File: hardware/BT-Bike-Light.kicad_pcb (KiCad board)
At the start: 4 copper layers, 35 x 80 mm, 46 parts, among them J101 USB_C_Charge_Port, J102 Conn_ARM_SWD_TagConnect_TC203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, J103 BATT, Q101 DMN3731U-7, SW102 Button, U101 BT840, U102 nPM1300, U103 FEM11-F09, U105 TPS92201

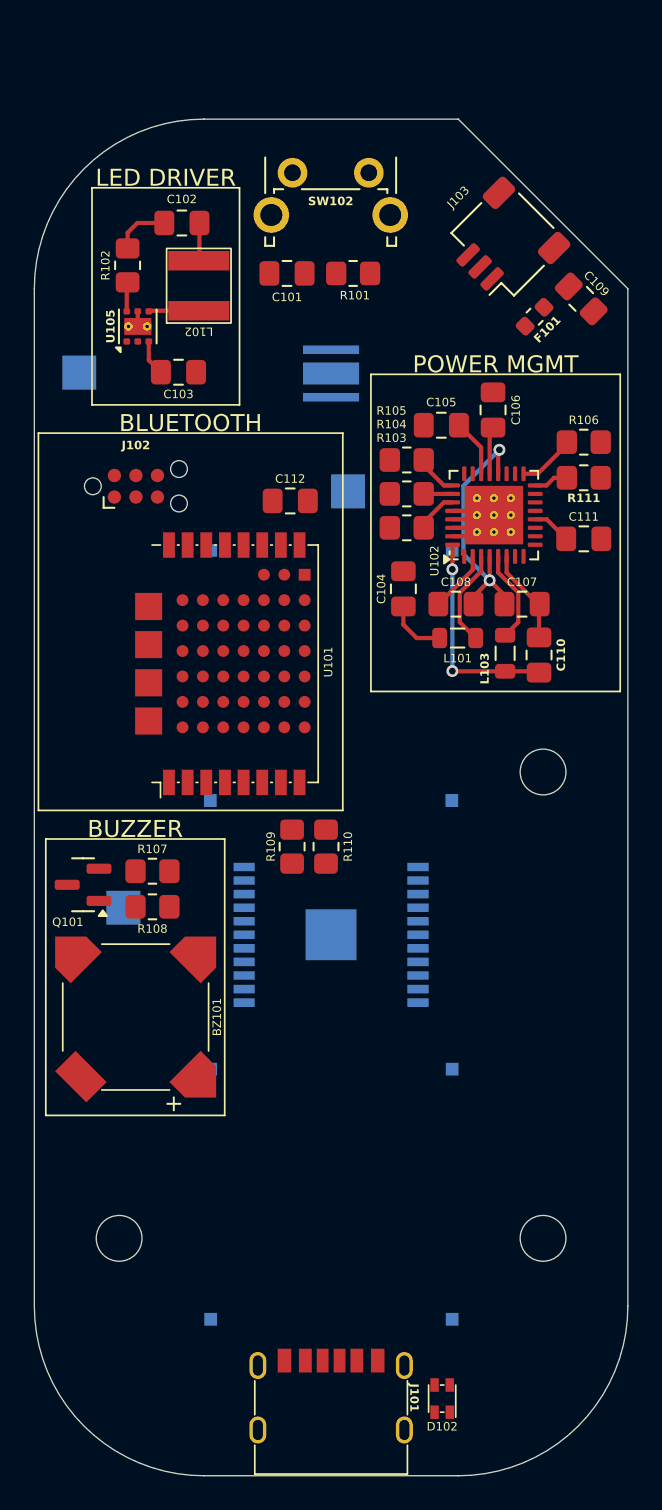
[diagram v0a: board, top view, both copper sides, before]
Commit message: Schematic cleanup
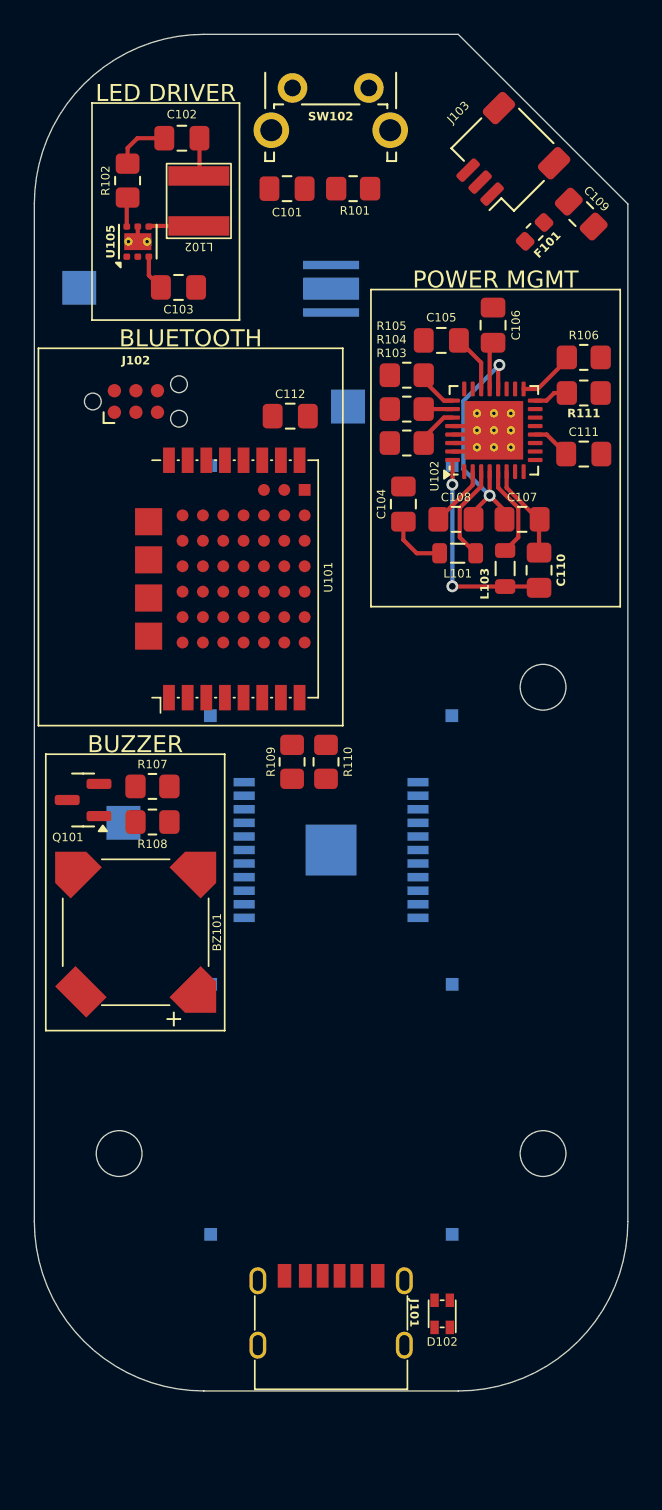
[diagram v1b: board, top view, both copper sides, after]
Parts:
- moved BZ101 5.00 mm to (131.0, 113.0)
- moved C101 5.00 mm to (139.9, 69.1)
- moved C102 5.00 mm to (133.7, 66.1)
- moved C103 5.00 mm to (133.5, 74.9)
- moved C104 5.00 mm to (146.8, 87.7)
- moved C105 5.00 mm to (149.0, 78.0)
- moved C106 5.00 mm to (152.1, 77.2)
- moved C107 5.00 mm to (153.8, 88.6)
- moved C108 5.00 mm to (149.9, 88.6)
- moved C109 5.00 mm to (157.2, 70.6)
- moved C110 5.00 mm to (154.8, 91.6)
- moved C111 5.00 mm to (157.4, 84.8)
- moved C112 5.00 mm to (140.1, 82.5)
- moved D101 5.00 mm to (142.5, 75.0)
- moved D102 5.00 mm to (149.1, 135.4)
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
